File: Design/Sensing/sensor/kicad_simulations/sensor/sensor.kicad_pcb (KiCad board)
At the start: 2 copper layers, 44 parts, among them J1 Conn_02x14_Counter_Clockwise, J11 Conn_01x01_Pin, J12 Conn_01x02_Pin, J15 Conn_01x02_Pin, J16 Conn_01x01_Pin, J17 Conn_01x02_Pin, J18 Conn_01x01_Pin, J4 Conn_01x02_Pin, J6 Conn_01x01_Pin, J7 Conn_01x02_Pin, J9 Conn_01x02_Pin, Q1 MMBT2222A, Q2 MMBT2222A, Q3 MMBT2222A, U1 TSSP58038, U2 TSSP58038, U3 TSSP58038, U4 BUF602xD, U5 BUF602xD, U6 BUF602xD

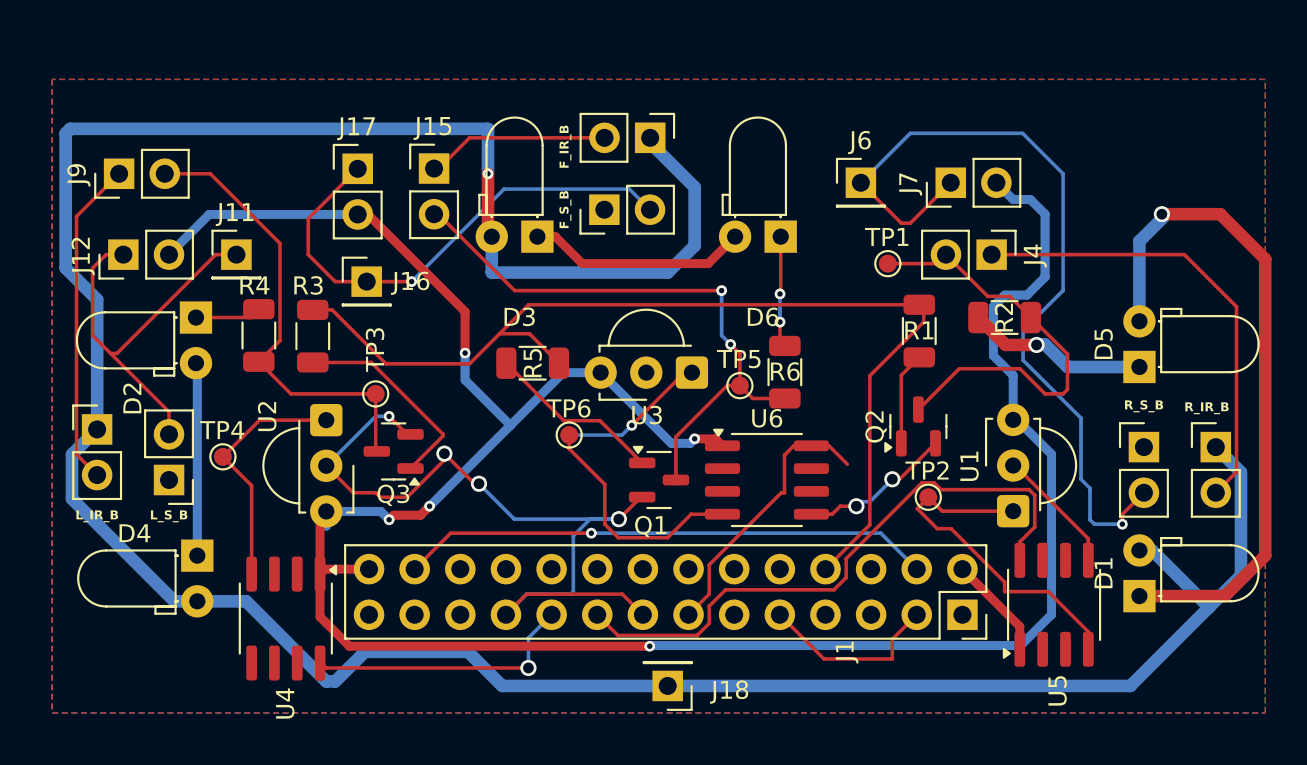
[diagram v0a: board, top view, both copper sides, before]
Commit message: pcb placement redo
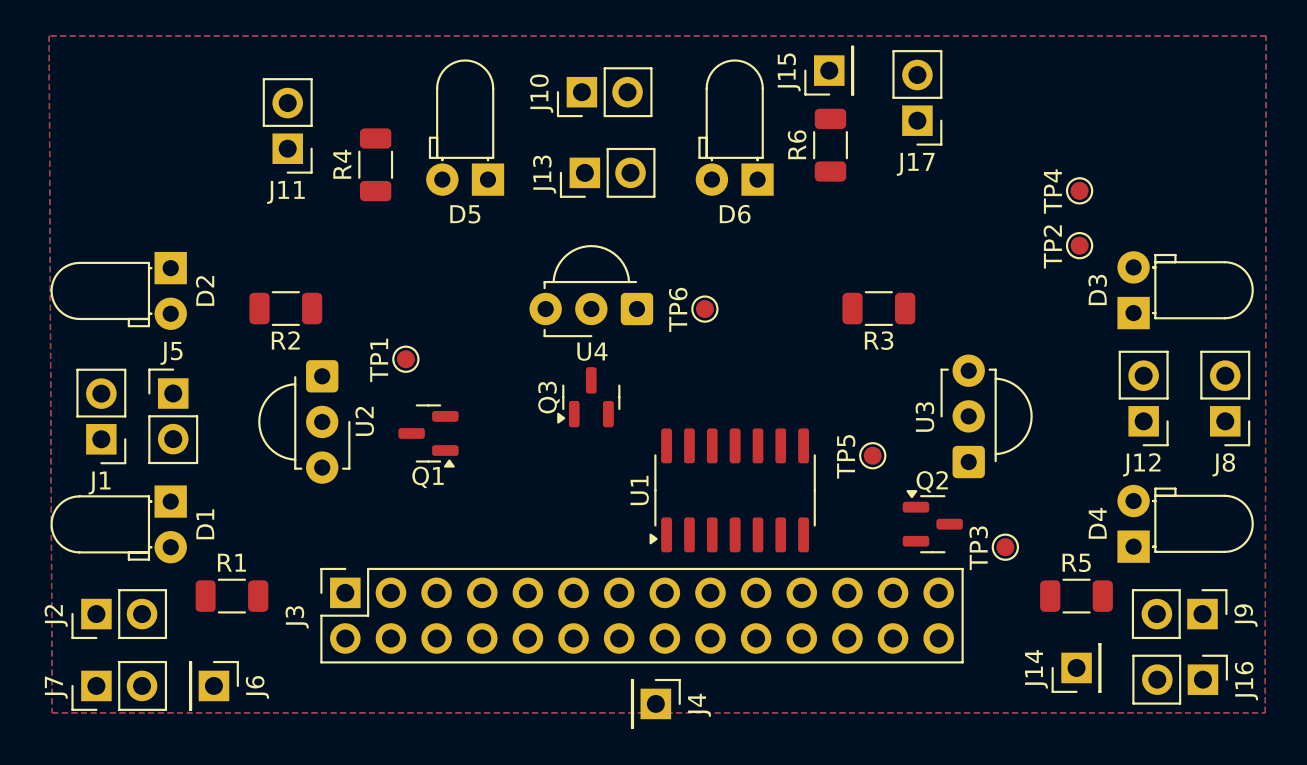
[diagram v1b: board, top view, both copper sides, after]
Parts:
- removed F_IR_B, F_S_B, L_IR_B, L_S_B, R_IR_B, R_S_B: Conn_01x02_Pin, Connector_PinHeader_2.54mm:PinHeader_1x02_P2.54mm_Vertical
- removed J18: Conn_01x01_Pin, Connector_PinHeader_2.54mm:PinHeader_1x01_P2.54mm_Vertical
- removed U5, U6: BUF602xD, Package_SO:SOIC-8_3.9x4.9mm_P1.27mm
- added J10: Conn_01x02_Pin, Connector_PinHeader_2.54mm:PinHeader_1x02_P2.54mm_Vertical, F.Cu at (113.5, 94.0)
- added J13: Conn_01x02_Pin, Connector_PinHeader_2.54mm:PinHeader_1x02_P2.54mm_Vertical, F.Cu at (113.6, 98.5)
- added J14: Conn_01x01_Pin, Connector_PinHeader_2.54mm:PinHeader_1x01_P2.54mm_Vertical, F.Cu at (141.0, 126.0)
- added J2: Conn_01x02_Pin, Connector_PinHeader_2.54mm:PinHeader_1x02_P2.54mm_Vertical, F.Cu at (86.5, 123.0)
- added J3: Conn_02x14_Counter_Clockwise, Connector_PinSocket_2.54mm:PinSocket_2x14_P2.54mm_Vertical, F.Cu at (100.3, 121.8)
- added J5: L_S_B, Connector_PinHeader_2.54mm:PinHeader_1x02_P2.54mm_Vertical, F.Cu at (90.7, 110.7)
- added J8: Conn_01x02_Pin, Connector_PinHeader_2.54mm:PinHeader_1x02_P2.54mm_Vertical, F.Cu at (149.3, 112.3)
- J1: value Conn_02x14_Counter_Clockwise -> Conn_01x02_Pin; footprint Connector_PinSocket_2.54mm:PinSocket_2x14_P2.54mm_Vertical -> Connector_PinHeader_2.54mm:PinHeader_1x02_P2.54mm_Vertical
- J11, J16: value Conn_01x01_Pin -> Conn_01x02_Pin; footprint Connector_PinHeader_2.54mm:PinHeader_1x01_P2.54mm_Vertical -> Connector_PinHeader_2.54mm:PinHeader_1x02_P2.54mm_Vertical
- J15, J4: value Conn_01x02_Pin -> Conn_01x01_Pin; footprint Connector_PinHeader_2.54mm:PinHeader_1x02_P2.54mm_Vertical -> Connector_PinHeader_2.54mm:PinHeader_1x01_P2.54mm_Vertical
- Q1, Q2, Q3: value MMBT2222A -> MMBT5551L
- R4: value 18 -> 2.7k
- R5: value 2.7k -> 18
- U1: value TSSP58038 -> LM324; footprint OptoDevice:Vishay_MINICAST-3Pin -> Package_SO:SOIC-14_3.9x8.7mm_P1.27mm
- U4: value BUF602xD -> TSSP58038; footprint Package_SO:SOIC-8_3.9x4.9mm_P1.27mm -> OptoDevice:Vishay_MINICAST-3Pin
- moved J9 65.1 mm to (148.0, 123.0), turned to -90 degrees
- moved J12 57.5 mm to (144.7, 112.3), turned to 180 degrees
- moved J7 55.2 mm to (86.5, 127.0)
- moved D1 54.2 mm to (90.6, 116.7), turned to -90 degrees
- moved D4 52.1 mm to (144.2, 119.2), turned to 90 degrees
- moved J16 51.5 mm to (148.0, 126.7), turned to -90 degrees
- moved TP4 49.9 mm to (141.2, 99.5), turned to 90 degrees
- moved J1 48.9 mm to (86.7, 113.3), turned to 180 degrees
- moved J6 45.6 mm to (93.0, 127.0), turned to -90 degrees
- moved R1 41.0 mm to (94.0, 122.0), turned to 0 degrees
- moved R2 40.0 mm to (97.0, 106.0)
- moved D5 37.7 mm to (108.2, 98.8), turned to 180 degrees
- moved TP3 36.1 mm to (137.0, 119.3)
- moved D3 33.4 mm to (144.2, 106.2), turned to 90 degrees
- moved R5 32.9 mm to (141.0, 122.0)
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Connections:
- D2 pad 2: Net-(D2-A) -> Net-(D1-K)
- D4 pad 1: Net-(D2-A) -> Net-(D4-K)
- D4 pad 2: /5V -> Net-(D3-K)
- D5 pad 2: Net-(D1-K) -> /5V
- D6 pad 2: Net-(D3-K) -> Net-(D5-K)
- J1 pad 1: /RESV3 -> /5V
- J1 pad 2: /3V3 -> Net-(J1-Pin_2)
- J12 pad 1: Net-(J10-Pin_2) -> GND
- J12 pad 2: /3V3 -> Net-(J12-Pin_2)
- J15 pad 1: Net-(J14-Pin_2) -> Net-(J13-Pin_2)
- J16 pad 1: Net-(J13-Pin_2) -> Net-(J12-Pin_2)
- J4 pad 1: Net-(J3-Pin_2) -> /5V
- Q1 pad 3: Net-(J15-Pin_2) -> Net-(J2-Pin_2)
- Q2 pad 3: Net-(J4-Pin_2) -> Net-(J9-Pin_2)
- Q3 pad 3: Net-(J9-Pin_2) -> Net-(J11-Pin_2)
- R1 pad 1: Net-(Q2-B) -> Net-(Q1-B)
- R2 pad 1: Net-(J4-Pin_2) -> Net-(J2-Pin_2)
- R2 pad 2: Net-(D5-K) -> Net-(D2-K)
- R3 pad 1: Net-(Q3-B) -> Net-(Q2-B)
- R4 pad 1: Net-(J9-Pin_2) -> Net-(Q3-B)
- R4 pad 2: Net-(D2-K) -> /PE15
- R5 pad 1: Net-(Q1-B) -> Net-(J9-Pin_2)
- R5 pad 2: /PE15 -> Net-(D4-K)
- R6 pad 1: Net-(J15-Pin_2) -> Net-(J11-Pin_2)
- TP1 pad 1: Net-(J4-Pin_2) -> Net-(J2-Pin_2)
- TP2 pad 1: Net-(U1-OUT) -> Net-(U1A-+)
- TP4 pad 1: Net-(U2-OUT) -> Net-(J11-Pin_2)
- TP5 pad 1: Net-(J15-Pin_2) -> Net-(U1B-+)
- TP6 pad 1: Net-(U3-OUT) -> Net-(U1C-+)
- U1 pad 1: Net-(U1-OUT) -> /PC4
- U1 pad 2: GND -> /PC4
- U1 pad 3: /3V3 -> Net-(U1A-+)
- U2 pad 1: Net-(U2-OUT) -> Net-(U1A-+)
- U3 pad 1: Net-(U3-OUT) -> Net-(U1B-+)
- U4 pad 1: /3V3 -> Net-(U1C-+)
- U4 pad 2: unconnected-(U4-NC-Pad2) -> GND
- U4 pad 3: unconnected-(U4-NC-Pad3) -> /3V3
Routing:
- net /5V: track 159.0 -> 0.00 mm, vias 1 -> 0
- net /3V3: track 141.2 -> 0.00 mm, vias 5 -> 0
- net GND: track 72.6 -> 0.00 mm, vias 6 -> 0
- net /PE15: track 57.4 -> 0.00 mm
- net Net-(J5-Pin_2): track 46.1 -> 0.00 mm, vias 1 -> 0
- net Net-(D1-K): track 38.0 -> 0.00 mm, vias 1 -> 0
- net /PA7: track 33.8 -> 0.00 mm
- net Net-(J15-Pin_2): track 33.4 -> 0.00 mm, vias 2 -> 0
- net /BATT: track 29.6 -> 0.00 mm, vias 1 -> 0
- net Net-(J13-Pin_2): track 28.2 -> 0.00 mm, vias 1 -> 0
- net Net-(J3-Pin_2): track 25.7 -> 0.00 mm
- net Net-(J9-Pin_2): track 25.6 -> 0.00 mm
- net Net-(J4-Pin_2): track 24.4 -> 0.00 mm
- net Net-(J10-Pin_2): track 22.3 -> 0.00 mm
- net Net-(U3-OUT): track 21.4 -> 0.00 mm, vias 1 -> 0
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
